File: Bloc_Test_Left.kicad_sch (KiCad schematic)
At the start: 0 parts

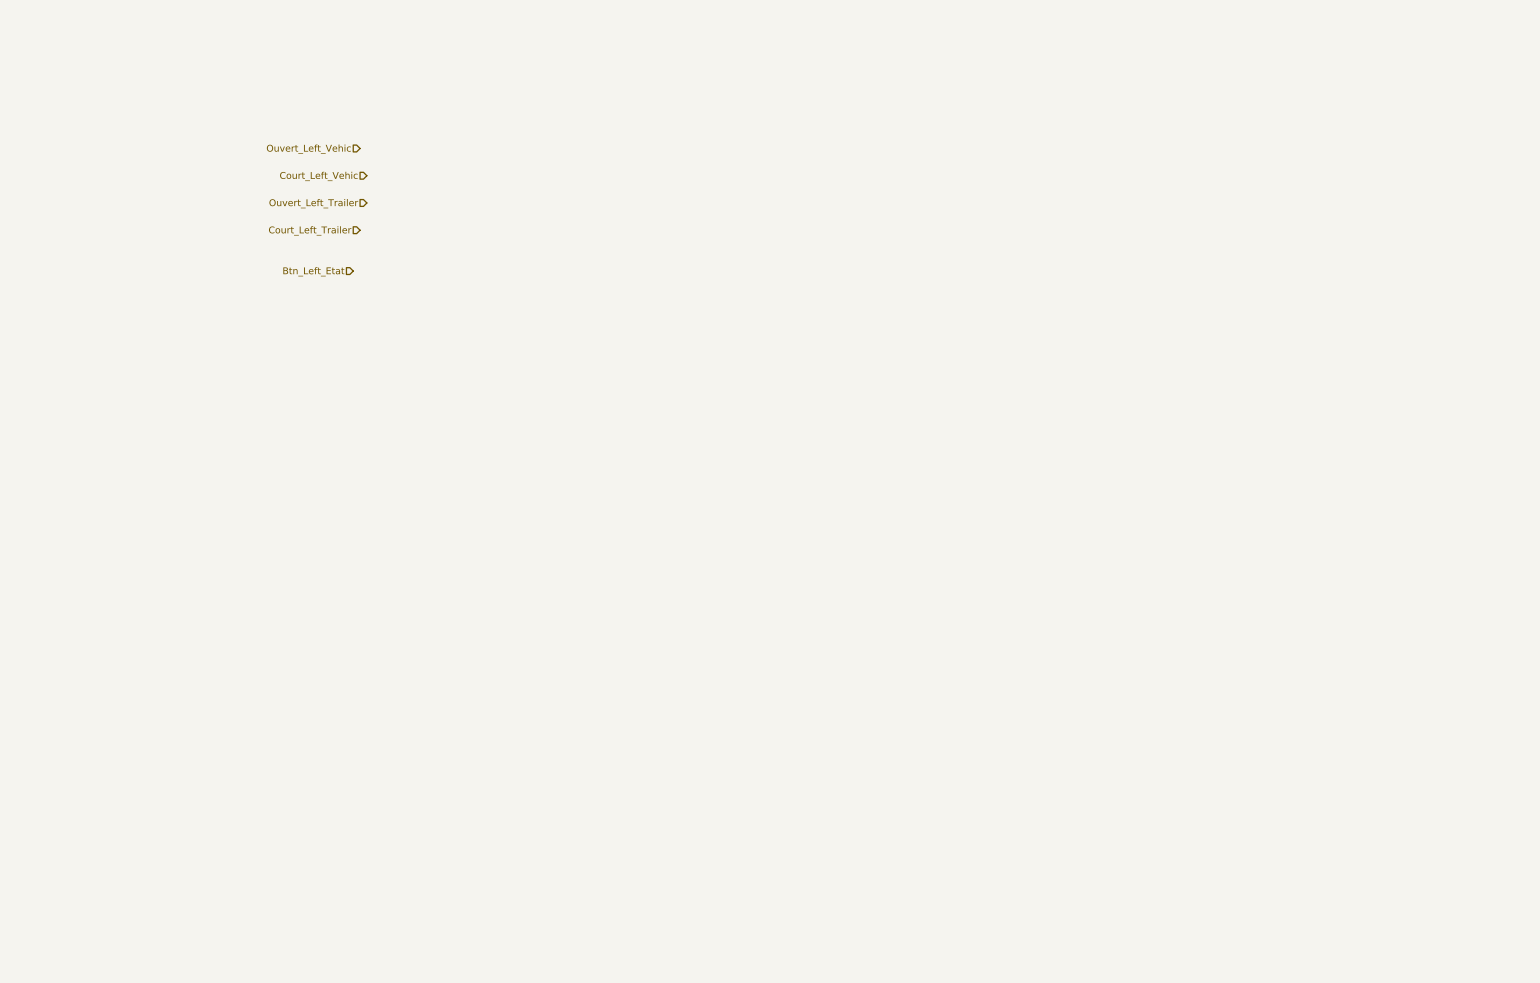
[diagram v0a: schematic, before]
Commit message: Add files via upload
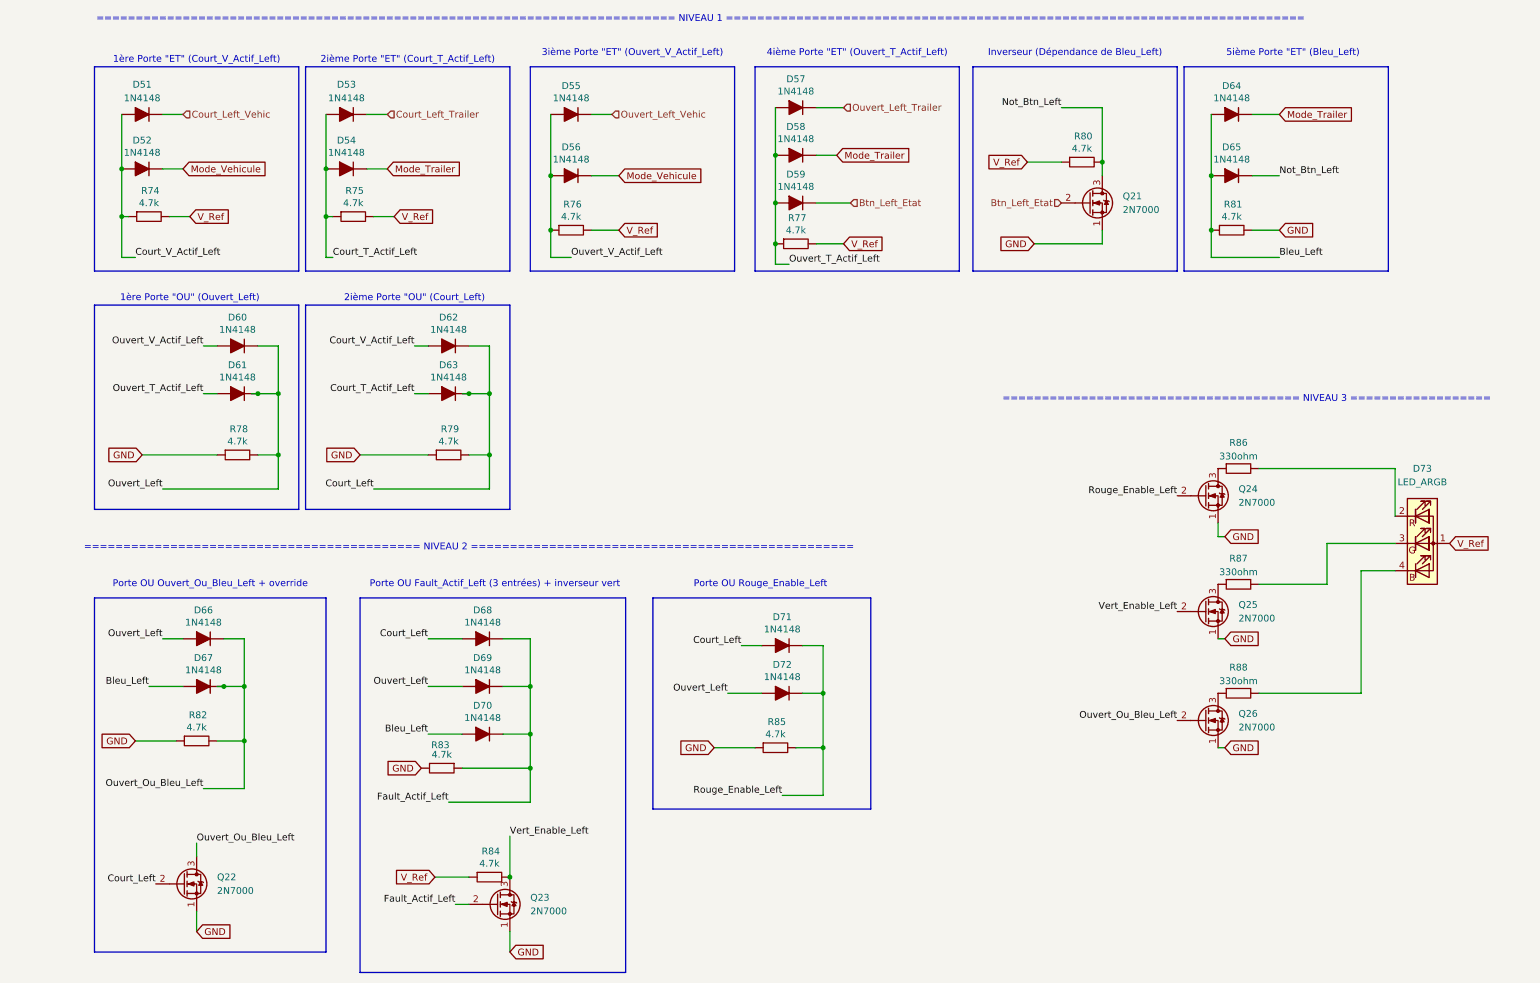
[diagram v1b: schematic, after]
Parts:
- added D51, D52, D53, D54, D55, D56, D57, D58, D59, D60, D61, D62, D63, D64, D65, D66, D67, D68, D69, D70, D71, D72: 1N4148, PCM_Diode_THT_AKL:D_DO-35_SOD27_P7.62mm_Horizontal, symbol PCM_Diode_AKL:1N4148
- added D73: LED_ARGB, symbol Device:LED_ARGB
- added Q21, Q22, Q23, Q24, Q25, Q26: 2N7000, Package_TO_SOT_THT:TO-92_Inline, symbol Transistor_FET:2N7000
- added R74, R75, R76, R77, R78, R79, R80, R81, R82, R83, R84, R85: 4.7k, Resistor_THT:R_Axial_DIN0207_L6.3mm_D2.5mm_P10.16mm_Horizontal, symbol PCM_SL_Resistors:4.7k
- added R86, R87, R88: 330ohm, Resistor_THT:R_Axial_DIN0207_L6.3mm_D2.5mm_P10.16mm_Horizontal, symbol PCM_SL_Resistors:330ohm
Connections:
- net Btn_Left_Etat: now also D59.1 (K), Q21.2 (G)
- net Court_Left_Trailer: now also D53.1 (K)
- net Court_Left_Vehic: now also D51.1 (K)
- net Ouvert_Left_Trailer: now also D57.1 (K)
- net Ouvert_Left_Vehic: now also D55.1 (K)
- new net: Q24.3 (D), R86.1
- new net: Q26.3 (D), R88.1
- new net: D73.4 (BK), R88.2
- new net: D73.2 (RK), R86.2
- new net: Q25.3 (D), R87.1
- new net: D73.3 (GK), R87.2
- new net Bleu_Left: D64.2 (A), D65.2 (A), D67.2 (A), D70.2 (A), R81.1
- new net Court_Left: D62.1 (K), D63.1 (K), D68.2 (A), D71.2 (A), Q22.2 (G), R79.2
- new net Court_T_Actif_Left: D53.2 (A), D54.2 (A), D63.2 (A), R75.1
- new net Court_V_Actif_Left: D51.2 (A), D52.2 (A), D62.2 (A), R74.1
- new net Fault_Actif_Left: D68.1 (K), D69.1 (K), D70.1 (K), Q23.2 (G), R83.1
- new net GND: Q21.1 (S), Q22.1 (S), Q23.1 (S), Q24.1 (S), Q25.1 (S), Q26.1 (S), R78.1, R79.1, R81.2, R82.1, R83.2, R85.1
- new net Mode_Trailer: D54.1 (K), D58.1 (K), D64.1 (K)
- new net Mode_Vehicule: D52.1 (K), D56.1 (K)
- new net Not_Btn_Left: D65.1 (K), Q21.3 (D), R80.2
- new net Ouvert_Left: D60.1 (K), D61.1 (K), D66.2 (A), D69.2 (A), D72.2 (A), R78.2
- new net Ouvert_Ou_Bleu_Left: D66.1 (K), D67.1 (K), Q22.3 (D), Q26.2 (G), R82.2
- new net Ouvert_T_Actif_Left: D57.2 (A), D58.2 (A), D59.2 (A), D61.2 (A), R77.1
- new net Ouvert_V_Actif_Left: D55.2 (A), D56.2 (A), D60.2 (A), R76.1
- new net Rouge_Enable_Left: D71.1 (K), D72.1 (K), Q24.2 (G), R85.2
- new net V_Ref: D73.1 (A), R74.2, R75.2, R76.2, R77.2, R80.1, R84.1
- new net Vert_Enable_Left: Q23.3 (D), Q25.2 (G), R84.2
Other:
- note added: "1ère Porte "ET" (Court_V_Actif_Left)"
- note added: "1ère Porte "OU" (Ouvert_Left)"
- note added: "2ième Porte "ET" (Court_T_Actif_Left)"
- note added: "2ième Porte "OU" (Court_Left)"
- note added: "3ième Porte "ET" (Ouvert_V_Actif_Left)"
- note added: "4ième Porte "ET" (Ouvert_T_Actif_Left)"
- note added: "5ième Porte "ET" (Bleu_Left)"
- note added: "====================================== NIVEAU 3 =================="
- note added: "=========================================== NIVEAU 2 ================================================="
- note added: "========================================================================== NIVEAU 1 =========================================================================="
- note added: "Inverseur (Dépendance de Bleu_Left)"
- note added: "Porte OU Fault_Actif_Left (3 entrées) + inverseur vert"
- note added: "Porte OU Ouvert_Ou_Bleu_Left + override"
- note added: "Porte OU Rouge_Enable_Left"

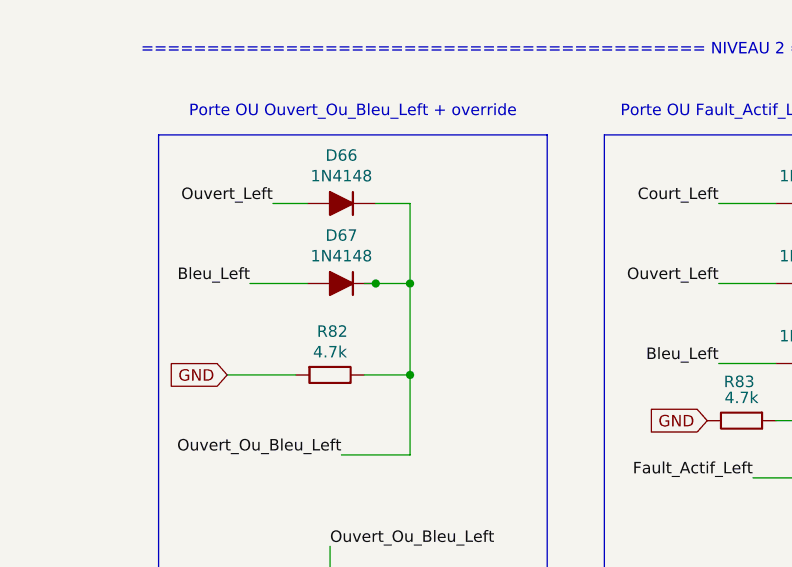
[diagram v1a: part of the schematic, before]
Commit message: Add files via upload
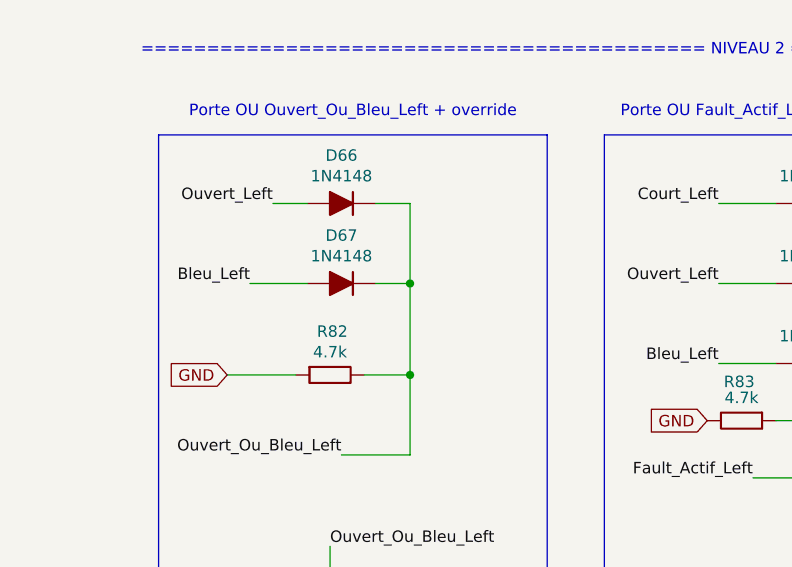
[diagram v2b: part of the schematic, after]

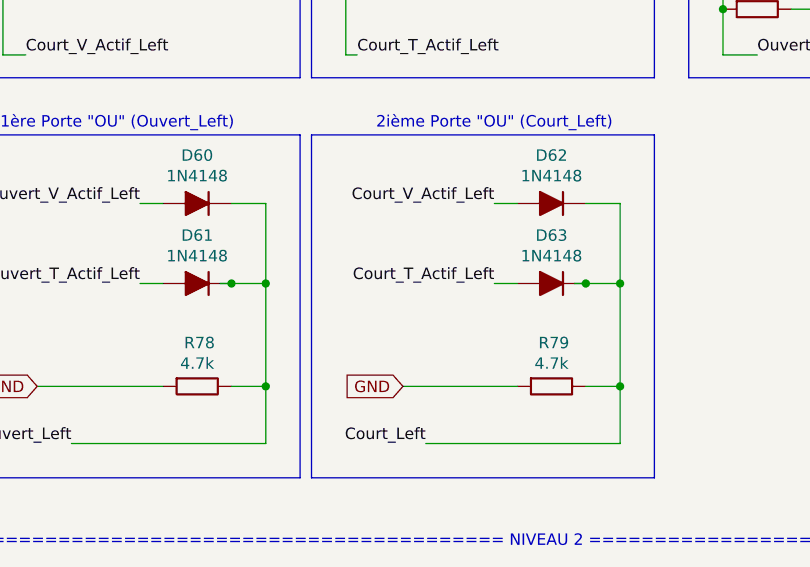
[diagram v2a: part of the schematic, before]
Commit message: Add files via upload
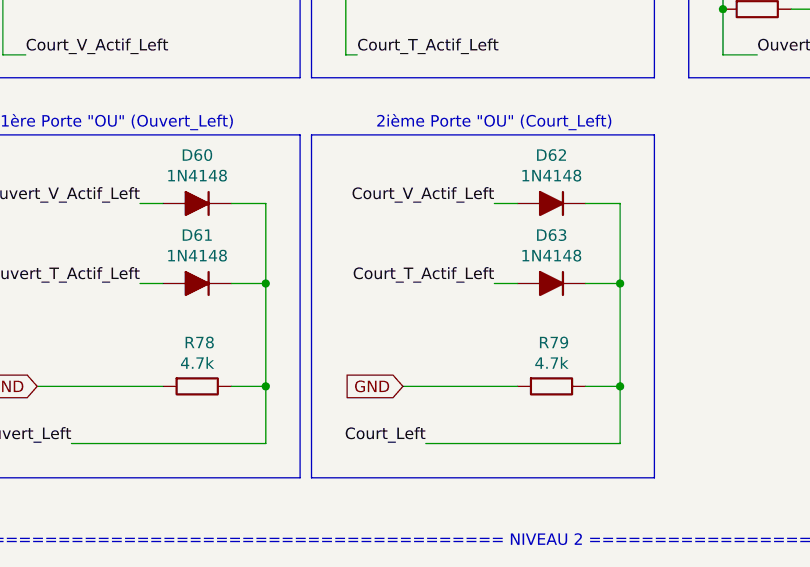
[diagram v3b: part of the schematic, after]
